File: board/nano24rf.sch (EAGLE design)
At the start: 20 parts

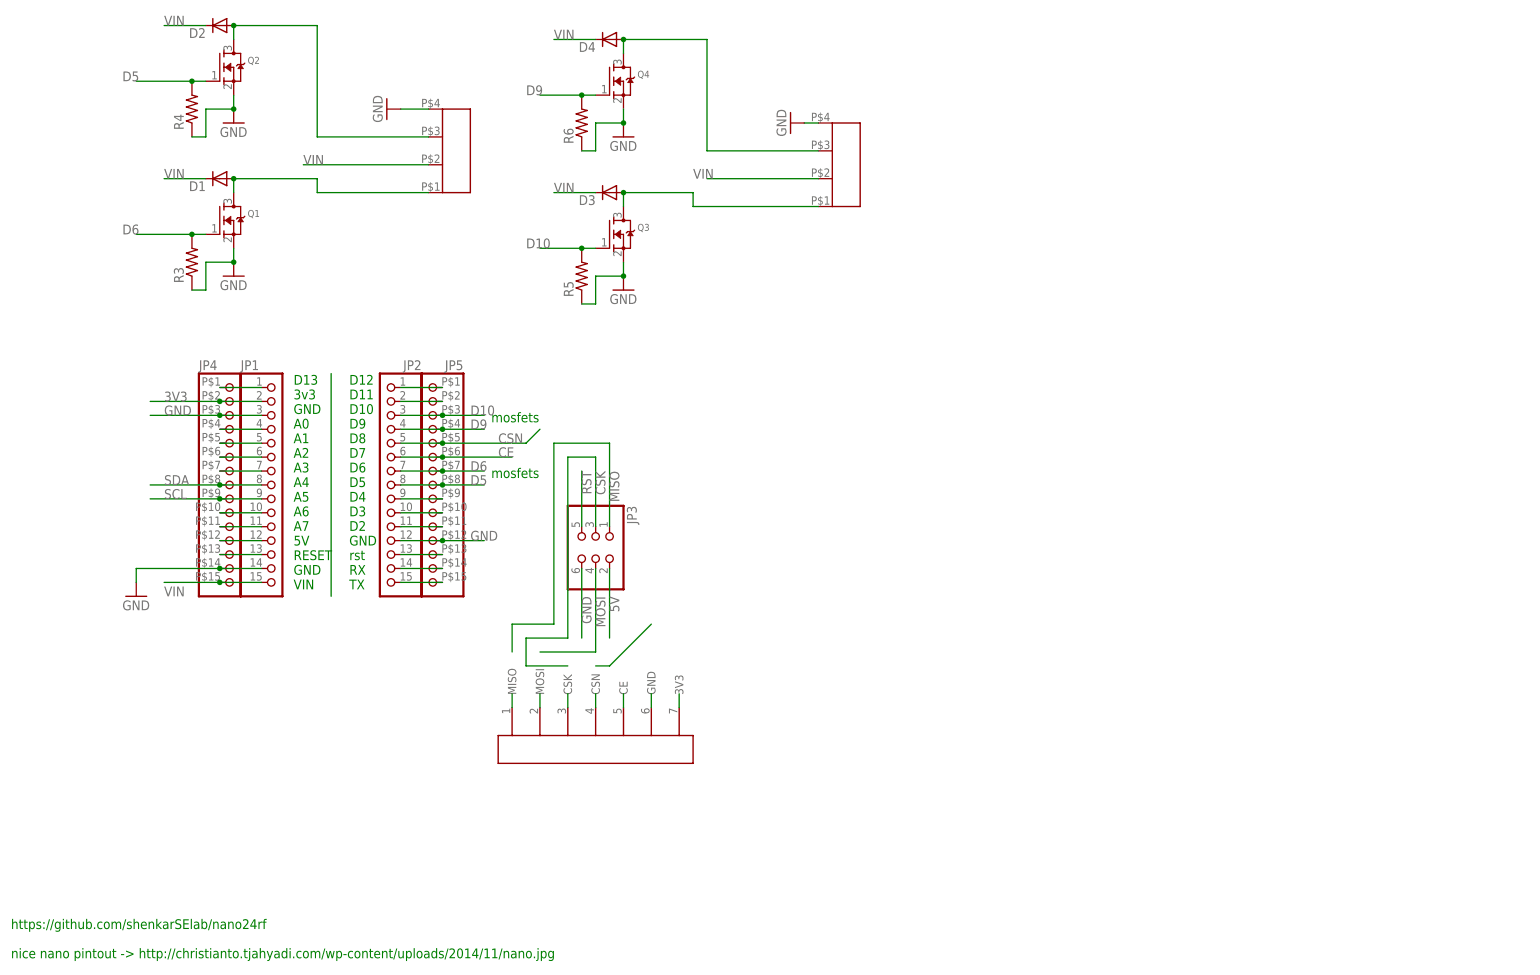
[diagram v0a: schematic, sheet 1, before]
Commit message: slight schema re-arange, and gerber
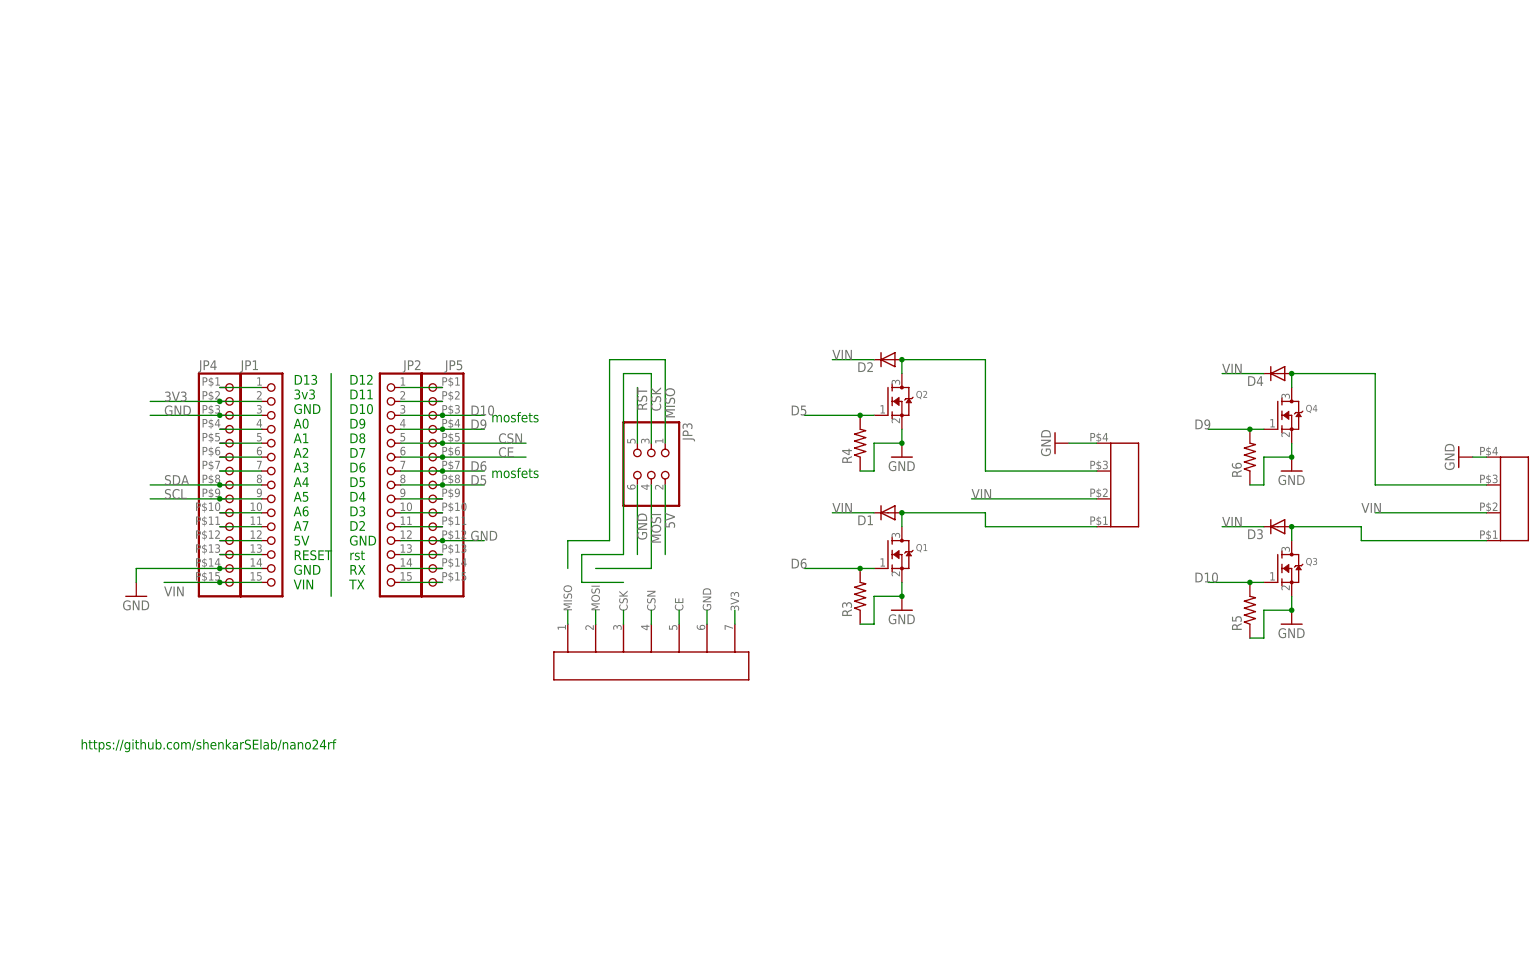
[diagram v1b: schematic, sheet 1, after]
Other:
- note added: "https://github.com/shenkarSElab/nano24rf"
- note removed: "https://github.com/shenkarSElab/nano24rf nice nano pintout -> http://christianto.tjahyadi.com/wp-content/uploads/2014/11/nano.jpg"
- moved on the sheet: D1, D2, D3, D4, JP3, Q1, Q2, Q3, Q4, R3, R4, R5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
